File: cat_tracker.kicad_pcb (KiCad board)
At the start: 2 copper layers, 42 x 46 mm, 32 parts, among them J1 Conn_01x02, J2 ISP, SW1 EN Btn, SW2 EN Btn, U1 NCP187, U2 USB_CType_6Pin, U3 MCP73831, U4 ESP32-WROOM-32E, U5 MPU-6050

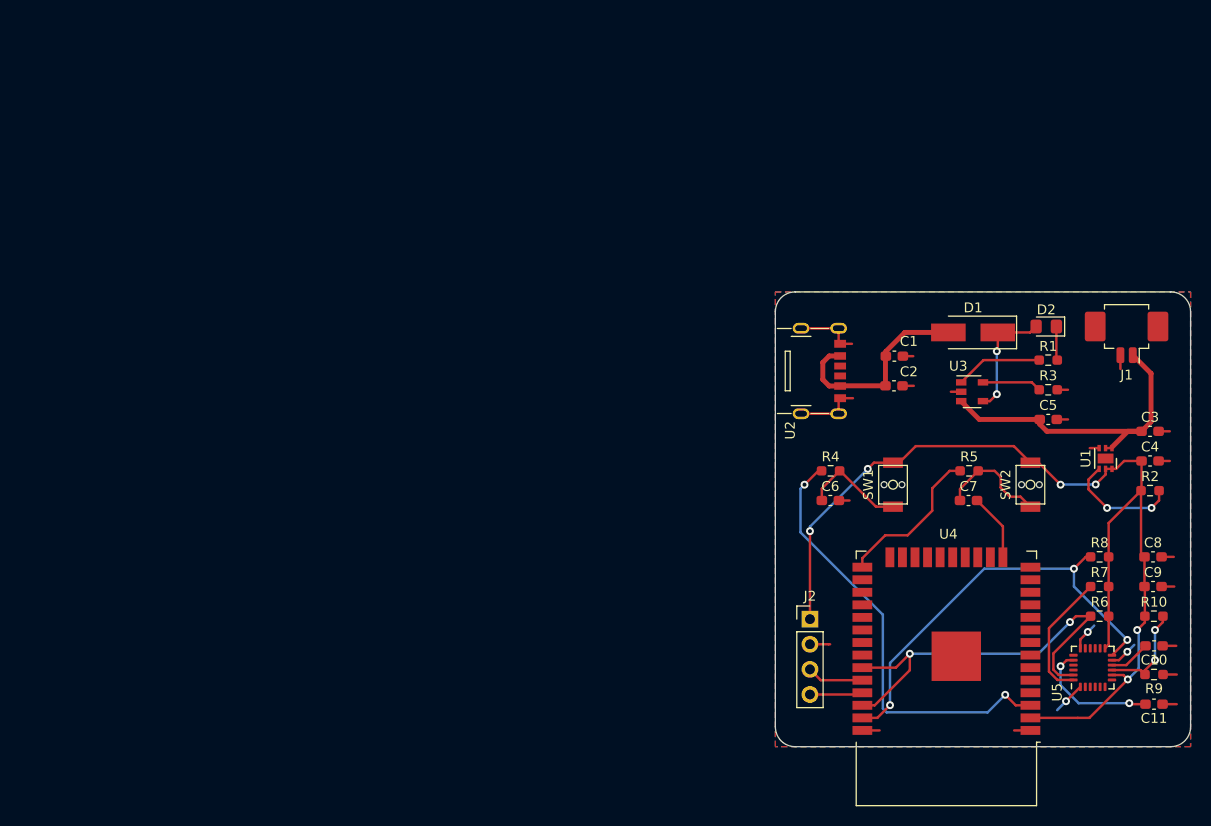
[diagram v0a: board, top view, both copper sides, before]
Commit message: 2021-09-08
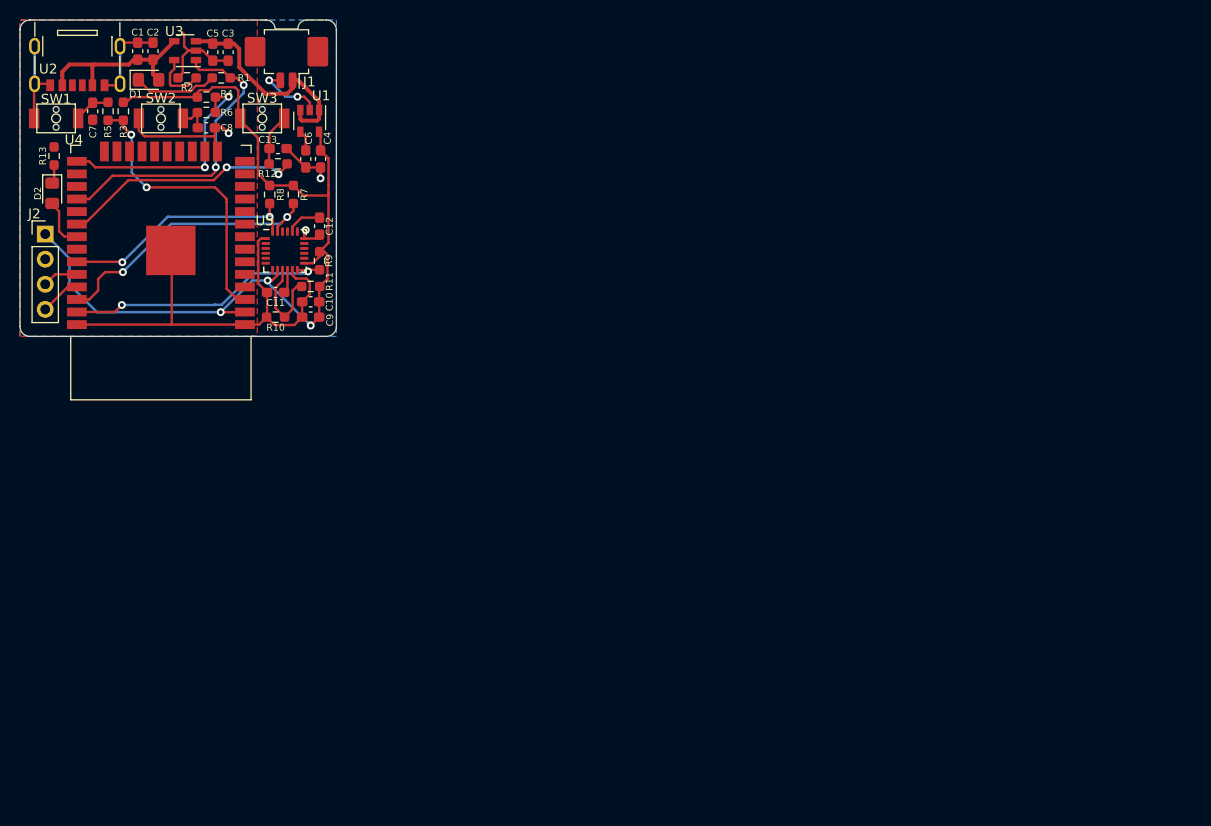
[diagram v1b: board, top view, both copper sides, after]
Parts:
- added C12: 2.2n, Capacitor_SMD:C_0603_1608Metric_Pad1.08x0.95mm_HandSolder, F.Cu at (30.3, 20.9)
- added C13: 100n, Capacitor_SMD:C_0603_1608Metric_Pad1.08x0.95mm_HandSolder, F.Cu at (26.1, 13.0)
- added R11: NC, Resistor_SMD:R_0603_1608Metric_Pad0.98x0.95mm_HandSolder, F.Cu at (29.4, 26.9)
- added R12: 1k, Resistor_SMD:R_0603_1608Metric_Pad0.98x0.95mm_HandSolder, F.Cu at (26.1, 14.6)
- added R13: 510, Resistor_SMD:R_0603_1608Metric_Pad0.98x0.95mm_HandSolder, F.Cu at (3.45, 13.8)
- added SW3: EN Btn, ali_Switch:NW3-A03-05, F.Cu at (24.5, 9.95)
- C11: value 2.2n -> 100n
- C4: value 10u -> 0.1u
- C6: value 100n -> 0.01u
- C8: value 10n -> 100n
- C9: value 100n -> 10n
- D1: value SK24/SMA -> LED/2012; footprint Diode_SMD:D_SMA_Handsoldering -> LED_SMD:LED_0805_2012Metric_Pad1.15x1.40mm_HandSolder
- R10: value NC -> 0
- R2: value 100k -> 2k
- R3: value 2k -> 100k
- R4: value 1k -> 100k
- R5: value 1k -> 100
- R6: value 10k -> 1k
- R9: value 0 -> 10k
- U1: value NCP187 -> MIC5318-3.3YD5-TR; footprint Package_DFN_QFN:DFN-6-1EP_2x2mm_P0.65mm_EP1x1.6mm -> Package_TO_SOT_SMD:SOT-23-5
- moved R2 106.0 mm to (16.9, 5.85), turned to 180 degrees
- moved C8 105.1 mm to (18.9, 10.9)
- moved R6 103.7 mm to (18.9, 9.35), turned to 180 degrees
- moved D2 101.4 mm to (3.25, 17.5), turned to 270 degrees
- moved C3 100.8 mm to (21.1, 3.25), turned to 270 degrees
- moved C11 98.1 mm to (25.9, 27.6), turned to 0 degrees
- moved R3 97.7 mm to (10.4, 9.23), turned to 90 degrees
- moved C7 96.9 mm to (7.35, 9.23), turned to 270 degrees
- moved SW2 95.4 mm to (14.2, 9.95), turned to 180 degrees
- moved R5 94.4 mm to (8.90, 9.23), turned to 90 degrees
- moved R9 94.2 mm to (30.3, 24.4), turned to 90 degrees
- moved R10 93.8 mm to (25.9, 30.1)
- moved SW1 92.4 mm to (3.65, 9.95), turned to 180 degrees
- moved C5 92.3 mm to (19.5, 3.25), turned to 270 degrees
- moved C10 92.1 mm to (29.4, 28.5)
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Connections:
- C10 pad 1: Earth -> +3V3
- C10 pad 2: Net-(C10-Pad2) -> Earth
- C8 pad 1: +3V3 -> Net-(C8-Pad1)
- D2 pad 2: Net-(D1-Pad1) -> LED
- R1 pad 1: Net-(D2-Pad1) -> Net-(D1-Pad1)
- R1 pad 2: Net-(R1-Pad2) -> CHRG
- R10 pad 1: +3V3 -> Earth
- R2 pad 1: +3V3 -> Net-(R2-Pad1)
- R2 pad 2: Net-(R2-Pad2) -> Earth
- R3 pad 1: Net-(R3-Pad1) -> EN
- R3 pad 2: Earth -> +3V3
- R4 pad 1: EN -> BOOT
- R4 pad 2: Net-(C6-Pad1) -> +3V3
- R5 pad 1: BOOT -> EN
- R6 pad 1: SCL -> BOOT
- R6 pad 2: +3V3 -> Net-(C8-Pad1)
- R7 pad 1: Net-(R7-Pad1) -> SCL
- R8 pad 1: INT -> SDA
- R9 pad 1: Earth -> INT
- R9 pad 2: Net-(R10-Pad2) -> +3V3
- SW1 pad 1: +3V3 -> Earth
- SW1 pad 2: Net-(C6-Pad1) -> Net-(C7-Pad1)
- SW2 pad 1: +3V3 -> Earth
- SW2 pad 2: Net-(C7-Pad1) -> Net-(C8-Pad1)
- U1 pad 2: BATT -> Earth
- U1 pad 3: Earth -> BATT
- U1 pad 4: Net-(R2-Pad2) -> Net-(C6-Pad1)
- U3 pad 1: Net-(R1-Pad2) -> CHRG
- U3 pad 4: Net-(D1-Pad1) -> VBUS
- U3 pad 5: Net-(R3-Pad1) -> Net-(R2-Pad1)
- U4 pad 28: Net-(U4-Pad28) -> CHRG
- U4 pad 30: Net-(U4-Pad30) -> BTN
- U4 pad 31: Net-(U4-Pad31) -> LED
- U4 pad 33: SCL -> SDA
- U5 pad 10: Net-(C10-Pad2) -> Net-(C11-Pad2)
- U5 pad 20: Net-(C11-Pad2) -> Net-(C12-Pad2)
- U5 pad 24: Net-(R7-Pad1) -> SDA
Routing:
- net Earth: track 54.0 -> 103.2 mm, vias 3 -> 5
- net CHRG: track 0.00 -> 31.4 mm, vias 0 -> 2
- net BTN: track 0.00 -> 24.5 mm, vias 0 -> 2
- net SDA: track 0.00 -> 24.4 mm, vias 0 -> 2
- net INT: track 44.0 -> 27.5 mm, vias 3 -> 2
- net EN: track 44.8 -> 29.3 mm
- net SCL: track 42.4 -> 28.9 mm
- net Net-(R7-Pad1): track 13.2 -> 0.00 mm
- net Net-(R2-Pad2): track 11.7 -> 0.00 mm, vias 2 -> 0
- net +3V3: track 103.8 -> 93.2 mm, vias 6 -> 3
- net BATT: track 33.3 -> 22.7 mm
- net Net-(C11-Pad2): track 12.9 -> 2.39 mm, vias 2 -> 0
- net Net-(R1-Pad2): track 8.82 -> 0.00 mm
- net Net-(C6-Pad1): track 10.6 -> 2.12 mm
- net BOOT: track 15.8 -> 24.3 mm, vias 0 -> 2
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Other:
- board size 42 x 46 mm -> 32 x 32 mm
- net class pwr: clearance 0.4 -> 0.35; trace_width 0.5 -> 0.4
- board text added: "Cat Tracker v0.2"

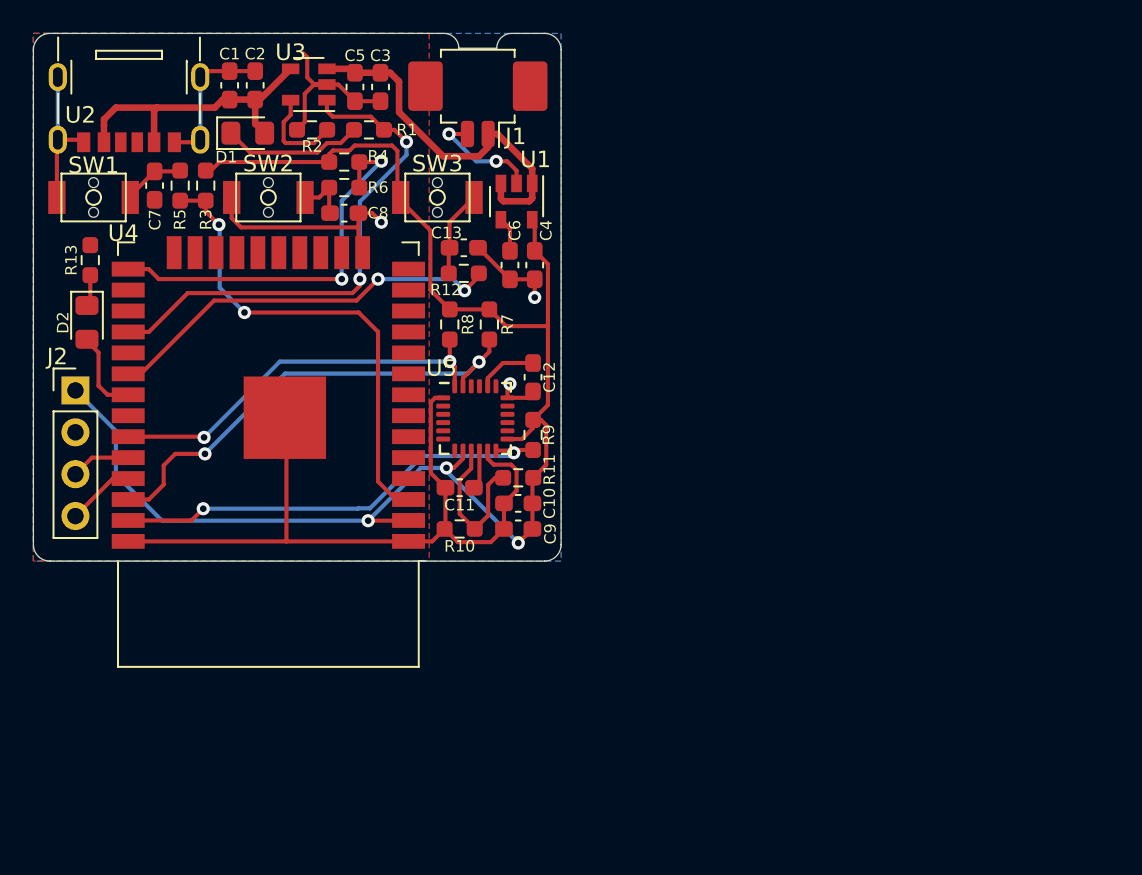
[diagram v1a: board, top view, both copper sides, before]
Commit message: 2021-12-14
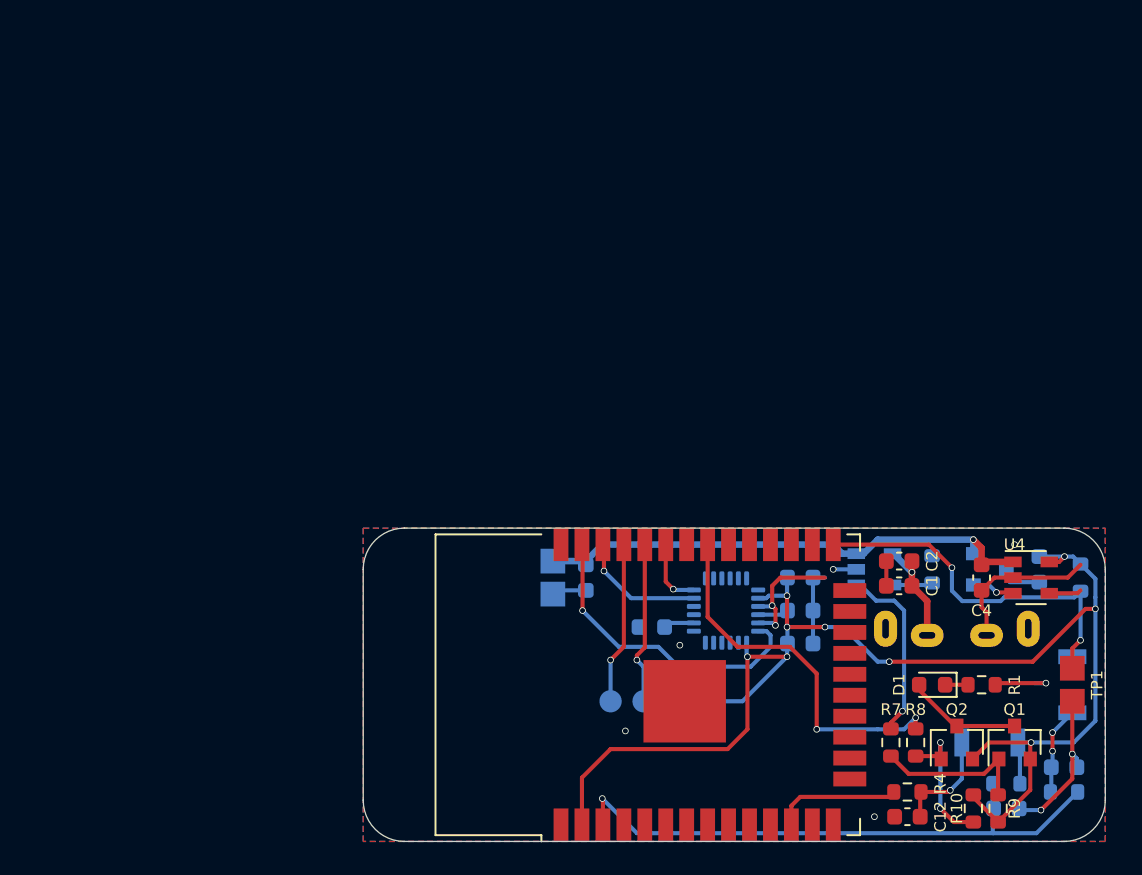
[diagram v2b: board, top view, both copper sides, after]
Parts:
- removed C6: 0.01u, Capacitor_SMD:C_0603_1608Metric_Pad1.08x0.95mm_HandSolder
- removed D2: LED/2012, LED_SMD:LED_0805_2012Metric_Pad1.15x1.40mm_HandSolder
- removed R11: NC, Resistor_SMD:R_0603_1608Metric_Pad0.98x0.95mm_HandSolder
- removed R12: 1k, Resistor_SMD:R_0603_1608Metric_Pad0.98x0.95mm_HandSolder
- removed R13: 510, Resistor_SMD:R_0603_1608Metric_Pad0.98x0.95mm_HandSolder
- removed SW3: EN Btn, ali_Switch:NW3-A03-05
- added Q1: pnp, Package_TO_SOT_SMD:SOT-23, F.Cu at (59.5, 43.0)
- added Q2: pnp, Package_TO_SOT_SMD:SOT-23, F.Cu at (56.0, 43.0)
- added TP1: , tp:boot, F.Cu at (63.0, 40.5)
- added U6: MPU-6050, Sensor_Motion:InvenSense_QFN-24_4x4mm_P0.5mm, B.Cu at (42.0, 35.0)
- C1, C2: footprint Capacitor_SMD:C_0603_1608Metric_Pad1.08x0.95mm_HandSolder -> Capacitor_SMD:C_0603_1608Metric
- C10, C7: footprint Capacitor_SMD:C_0603_1608Metric_Pad1.08x0.95mm_HandSolder -> Capacitor_SMD:C_0603_1608Metric; moved to B.Cu
- C11: value 100n -> 2.2n; footprint Capacitor_SMD:C_0603_1608Metric_Pad1.08x0.95mm_HandSolder -> Capacitor_SMD:C_0603_1608Metric; moved to B.Cu
- C12: value 2.2n -> 100n; footprint Capacitor_SMD:C_0603_1608Metric_Pad1.08x0.95mm_HandSolder -> Capacitor_SMD:C_0603_1608Metric
- C13: value 100n -> 1u; footprint Capacitor_SMD:C_0603_1608Metric_Pad1.08x0.95mm_HandSolder -> Capacitor_SMD:C_0603_1608Metric; moved to B.Cu
- C3: value 100n -> 10u; footprint Capacitor_SMD:C_0603_1608Metric_Pad1.08x0.95mm_HandSolder -> Capacitor_SMD:C_0603_1608Metric; moved to B.Cu
- C4: value 0.1u -> 100n; footprint Capacitor_SMD:C_0603_1608Metric_Pad1.08x0.95mm_HandSolder -> Capacitor_SMD:C_0603_1608Metric
- C5: value 10u -> 100n; footprint Capacitor_SMD:C_0603_1608Metric_Pad1.08x0.95mm_HandSolder -> Capacitor_SMD:C_0603_1608Metric; moved to B.Cu
- C8: value 100n -> 10n; footprint Capacitor_SMD:C_0603_1608Metric_Pad1.08x0.95mm_HandSolder -> Capacitor_SMD:C_0603_1608Metric; moved to B.Cu
- C9: value 10n -> 100n; footprint Capacitor_SMD:C_0603_1608Metric_Pad1.08x0.95mm_HandSolder -> Capacitor_SMD:C_0603_1608Metric; moved to B.Cu
- D1: value LED/2012 -> LED/1608; footprint LED_SMD:LED_0805_2012Metric_Pad1.15x1.40mm_HandSolder -> LED_SMD:LED_0603_1608Metric
- J1: footprint Connector_Molex:Molex_PicoBlade_53261-0271_1x02-1MP_P1.25mm_Horizontal -> tp:boot; moved to B.Cu
- J2: footprint Connector_PinHeader_2.54mm:PinHeader_1x04_P2.54mm_Vertical -> Connector_PinHeader_2.00mm:PinHeader_1x04_P2.00mm_Vertical; moved to B.Cu
- R1: footprint Resistor_SMD:R_0603_1608Metric_Pad0.98x0.95mm_HandSolder -> Resistor_SMD:R_0603_1608Metric
- R10: value 0 -> 33k; footprint Resistor_SMD:R_0603_1608Metric_Pad0.98x0.95mm_HandSolder -> Resistor_SMD:R_0603_1608Metric
- R2: footprint Resistor_SMD:R_0603_1608Metric_Pad0.98x0.95mm_HandSolder -> Resistor_SMD:R_0603_1608Metric; moved to B.Cu
- R3: value 100k -> 0; footprint Resistor_SMD:R_0603_1608Metric_Pad0.98x0.95mm_HandSolder -> Resistor_SMD:R_0603_1608Metric; moved to B.Cu
- R4: value 100k -> 1k; footprint Resistor_SMD:R_0603_1608Metric_Pad0.98x0.95mm_HandSolder -> Resistor_SMD:R_0603_1608Metric
- R5: value 100 -> 10k; footprint Resistor_SMD:R_0603_1608Metric_Pad0.98x0.95mm_HandSolder -> Resistor_SMD:R_0603_1608Metric; moved to B.Cu
- R6: value 1k -> 10k; footprint Resistor_SMD:R_0603_1608Metric_Pad0.98x0.95mm_HandSolder -> Resistor_SMD:R_0603_1608Metric; moved to B.Cu
- R7, R8, R9: value 10k -> 33k; footprint Resistor_SMD:R_0603_1608Metric_Pad0.98x0.95mm_HandSolder -> Resistor_SMD:R_0603_1608Metric
- SW1: footprint ali_Switch:NW3-A03-05 -> Button_Switch_SMD:SW_SPST_B3U-1000P; moved to B.Cu
- SW2: value EN Btn -> Btn; footprint ali_Switch:NW3-A03-05 -> Button_Switch_SMD:SW_SPST_B3U-1000P; moved to B.Cu
- U1: value MIC5318-3.3YD5-TR -> MCP100-315D; footprint Package_TO_SOT_SMD:SOT-23-5 -> Package_TO_SOT_SMD:SOT-23; moved to B.Cu
- U2: value USB_CType_6Pin -> USB_CType_2Pin; footprint ali_Connector:USB_CType_6Pin -> ali_Connector:USB_CType_2Pin; moved to B.Cu
- U3: moved to B.Cu
- U4: value ESP32-WROOM-32E -> MIC5318-3.3YD5-TR; footprint RF_Module:ESP32-WROOM-32 -> Package_TO_SOT_SMD:SOT-23-5
- U5: value MPU-6050 -> ESP32-WROOM-32E; footprint Sensor_Motion:InvenSense_QFN-24_4x4mm_P0.5mm -> RF_Module:ESP32-WROOM-32
- moved SW1 66.3 mm to (63.0, 39.5), turned to 270 degrees
- moved C7 65.5 mm to (62.5, 44.5), turned to 0 degrees
- moved R3 63.7 mm to (62.5, 46.0), turned to 180 degrees
- moved U2 62.0 mm to (56.0, 36.5)
- moved R5 61.9 mm to (59.0, 45.5), turned to 0 degrees
- moved SW2 54.8 mm to (58.0, 43.0)
- moved D1 53.3 mm to (54.5, 39.5), turned to 180 degrees
- moved R4 51.2 mm to (53.0, 46.0), turned to 0 degrees
- moved C5 50.8 mm to (61.0, 32.5)
- moved C1 50.7 mm to (52.5, 33.5), turned to 180 degrees
- moved R6 50.5 mm to (63.5, 33.0), turned to 90 degrees
- moved R1 50.1 mm to (57.5, 39.5)
- moved C2 48.6 mm to (52.5, 32.0), turned to 180 degrees
- moved U4 47.4 mm to (60.5, 33.0), turned to 0 degrees
- moved C13 47.3 mm to (59.0, 47.0)
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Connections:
- C10 pad 1: +3V3 -> Earth
- C10 pad 2: Earth -> Net-(C10-Pad2)
- C12 pad 1: Earth -> Net-(C12-Pad1)
- C12 pad 2: Net-(C12-Pad2) -> Earth
- C13 pad 1: Net-(C13-Pad1) -> EN
- C4 pad 1: +3V3 -> BATT
- C5 pad 1: BATT -> +3V3
- C8 pad 1: Net-(C8-Pad1) -> +3V3
- D1 pad 2: VBUS -> Net-(D1-Pad2)
- R1 pad 2: CHRG -> Earth
- R10 pad 1: Earth -> +3V3
- R10 pad 2: Net-(R10-Pad2) -> Net-(Q2-Pad1)
- R3 pad 2: +3V3 -> Net-(C7-Pad1)
- R4 pad 1: BOOT -> BTN
- R4 pad 2: +3V3 -> Net-(C12-Pad1)
- R5 pad 2: Net-(C7-Pad1) -> +3V3
- R6 pad 2: Net-(C8-Pad1) -> +3V3
- R7 pad 1: SCL -> Net-(Q1-Pad1)
- R7 pad 2: +3V3 -> CHRG
- R8 pad 1: SDA -> Net-(Q2-Pad1)
- R8 pad 2: +3V3 -> LED
- R9 pad 1: INT -> +3V3
- R9 pad 2: +3V3 -> Net-(Q1-Pad1)
- SW2 pad 1: Earth -> +3V3
- SW2 pad 2: Net-(C8-Pad1) -> Net-(C12-Pad1)
- U1 pad 1: BATT -> Net-(U1-Pad1)
- U1 pad 2: Earth -> BATT
- U1 pad 3: BATT -> Earth
- U4 pad 1: Earth -> BATT
- U4 pad 2: +3V3 -> Earth
- U4 pad 3: EN -> Net-(U1-Pad1)
- U4 pad 4: Net-(U4-Pad4) -> (no net)
- U4 pad 5: Net-(U4-Pad5) -> +3V3
- U5 pad 10: Net-(C11-Pad2) -> (no net)
- U5 pad 11: Earth -> (no net)
- U5 pad 12: INT -> BTN
- U5 pad 13: +3V3 -> (no net)
- U5 pad 15: (no net) -> Earth
- U5 pad 18: Earth -> (no net)
- U5 pad 2: (no net) -> +3V3
- U5 pad 20: Net-(C12-Pad2) -> (no net)
- U5 pad 23: SCL -> (no net)
- U5 pad 24: SDA -> (no net)
- U5 pad 3: (no net) -> EN
- U5 pad 6: Net-(U5-Pad6) -> (no net)
- U5 pad 7: Net-(U5-Pad7) -> (no net)
- U5 pad 8: +3V3 -> (no net)
- U5 pad 9: Net-(R10-Pad2) -> (no net)
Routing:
- net Earth: track 103.2 -> 43.2 mm, vias 5 -> 10
- net SCL: track 28.9 -> 7.76 mm, vias 2 -> 1
- net CHRG: track 31.4 -> 11.0 mm, vias 2 -> 1
- net SDA: track 24.4 -> 4.16 mm, vias 2 -> 1
- net LED: track 5.13 -> 22.8 mm, vias 0 -> 2
- net BTN: track 24.5 -> 7.72 mm, vias 2 -> 0
- net VBUS: track 18.4 -> 6.52 mm, vias 0 -> 1
- net Net-(Q1-Pad1): track 0.00 -> 9.56 mm
- net Net-(R10-Pad2): track 9.52 -> 0.00 mm
- net Net-(Q2-Pad1): track 0.00 -> 8.98 mm, vias 0 -> 2
- net BATT: track 22.7 -> 31.4 mm, vias 0 -> 1
- net INT: track 27.5 -> 18.9 mm, vias 2 -> 1
- net Net-(D1-Pad1): track 8.52 -> 1.39 mm
- net Net-(D1-Pad2): track 0.00 -> 7.01 mm
- net Net-(C12-Pad1): track 0.00 -> 6.53 mm, vias 0 -> 1
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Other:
- board size 32 x 32 mm -> 45 x 19 mm
- net class Default: via_dia 0.8 -> 0.4; via_drill 0.4 -> 0.3
- net class pwr: clearance 0.35 -> 0.2; via_dia 0.8 -> 0.4; via_drill 0.4 -> 0.3
- board text added: "+"
- board text added: "-"
- board text added: "g"
- board text added: "r"
- board text added: "t"
- board text added: "v"
- board text removed: "Cat Tracker v0.2"
